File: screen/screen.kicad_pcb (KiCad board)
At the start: 2 copper layers, 65 x 50 mm, 50 parts, among them P1 CONN_01X08, Q1 N_MOS, Q2 N_MOS, U1 uHDMI, U2 TFP401A, U3 TPS76333, U4 TSP61161, U5 M93C46, U6 HVT-4.3, U7 NHD-5.0

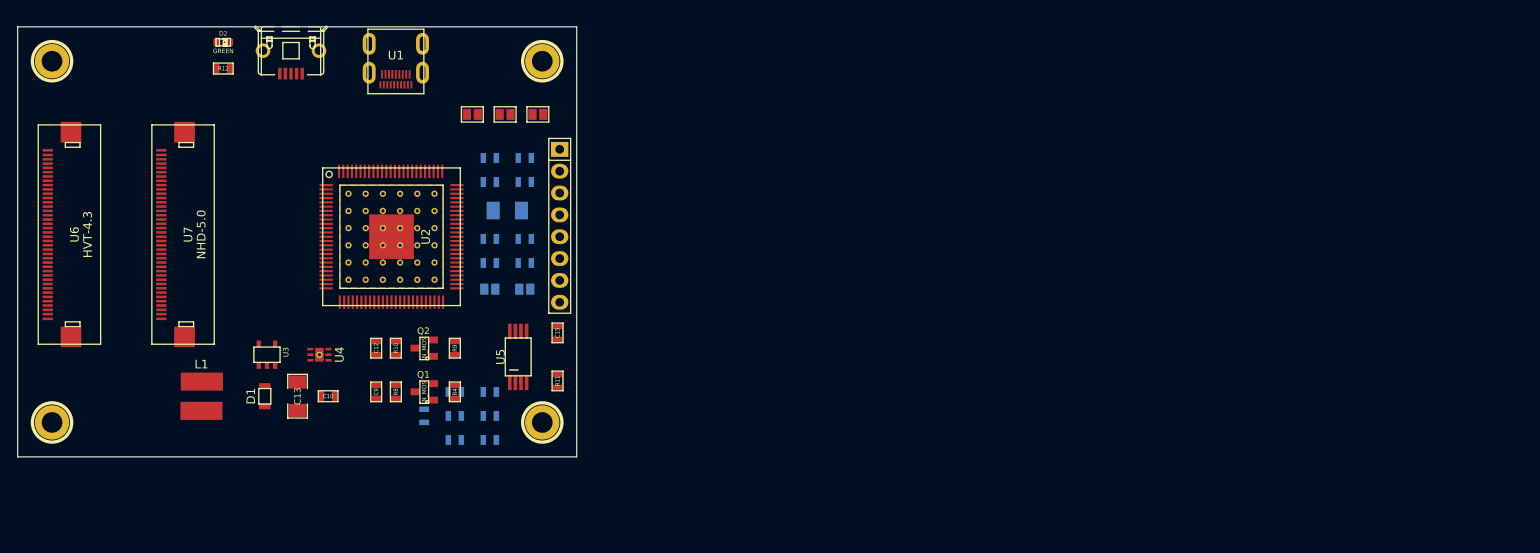
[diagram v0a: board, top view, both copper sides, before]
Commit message: moving around some stuff for routing
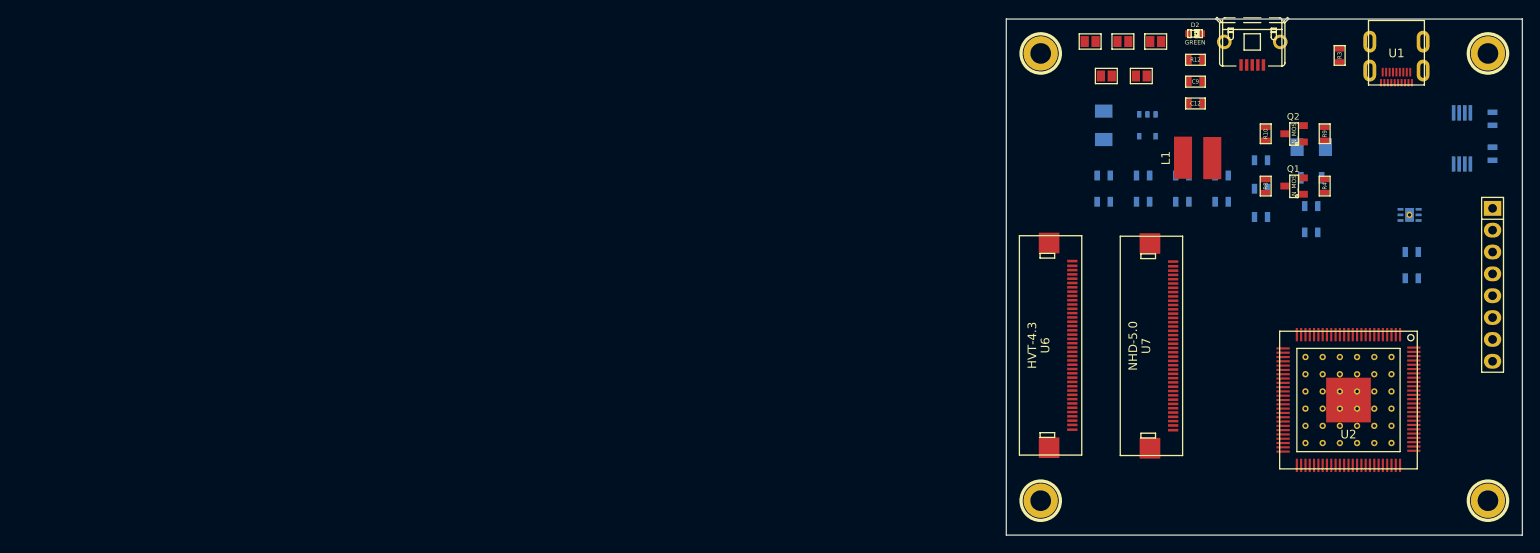
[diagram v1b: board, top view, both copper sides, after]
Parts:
- C10, C13, C15, D1, R11, U3, U4, U5: moved to B.Cu
- JP4, JP5, R3: moved to F.Cu
- moved U4 127.8 mm to (214.9, 80.8)
- moved D1 124.3 mm to (203.5, 76.5), turned to 0 degrees
- moved C13 121.4 mm to (203.5, 72.9), turned to 180 degrees
- moved L1 119.1 mm to (190.2, 74.2), turned to 90 degrees
- moved C10 116.4 mm to (203.5, 79.8), turned to 180 degrees
- moved U1 116.3 mm to (213.4, 58.9)
- moved 3PIN 115.3 mm to (172.0, 114.0)
- moved 1PIN 115.0 mm to (172.0, 62.0)
- moved R3 114.4 mm to (206.8, 62.2), turned to 270 degrees
- moved R12 113.0 mm to (190.0, 62.7)
- moved D2 113.0 mm to (189.9, 59.7)
- moved R11 112.9 mm to (224.5, 69.6), turned to 270 degrees
- moved U2 112.9 mm to (207.8, 102.3), turned to 180 degrees
- moved U5 112.6 mm to (221.0, 71.9), turned to 270 degrees
- moved R1 112.4 mm to (215.1, 85.1), turned to 180 degrees
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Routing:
- removed copper zone on F.Cu, net GND
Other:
- board size 65 x 50 mm -> 60 x 60 mm
